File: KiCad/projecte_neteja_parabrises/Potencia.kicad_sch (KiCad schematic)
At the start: 10 parts

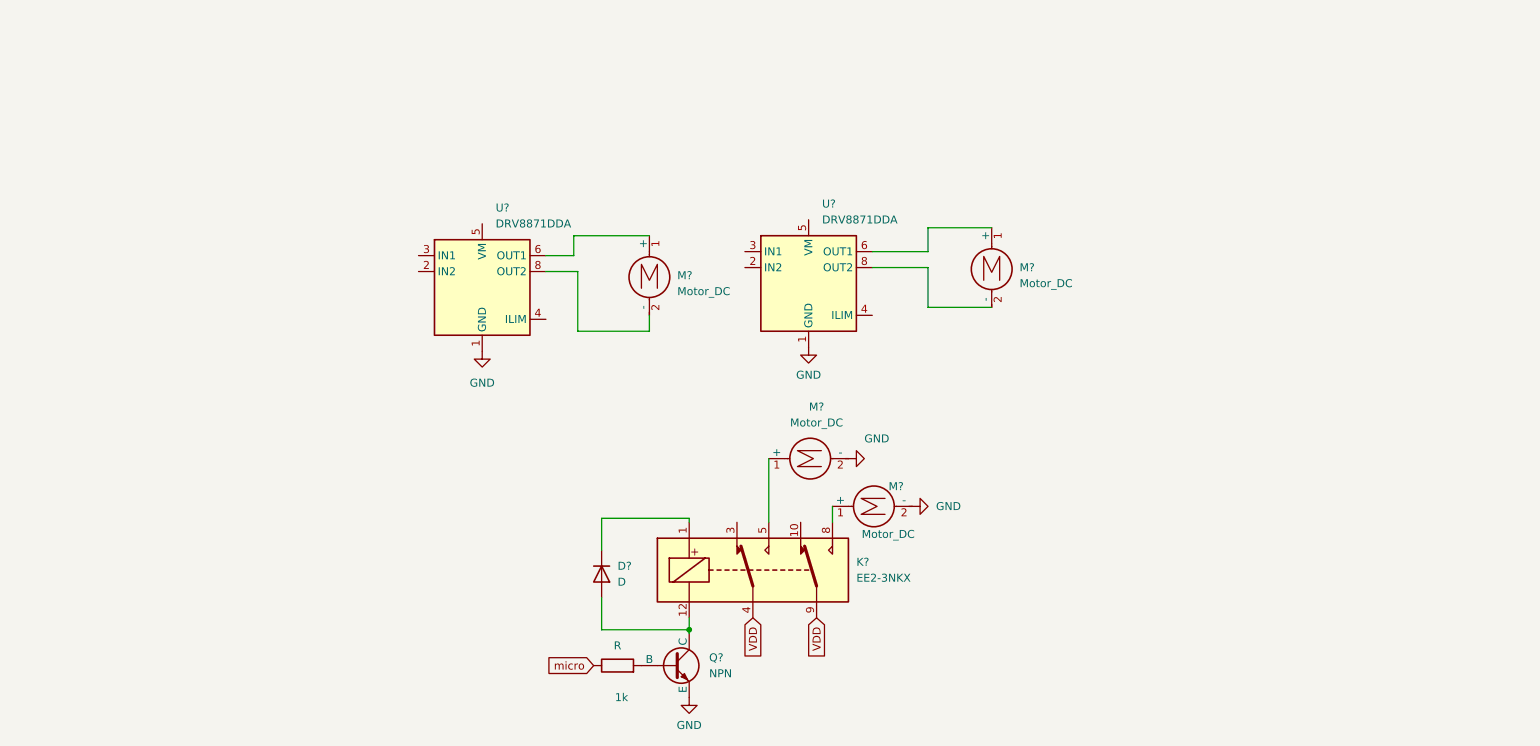
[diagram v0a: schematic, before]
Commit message: BOMBAS Y FINAL DEL CARRERA
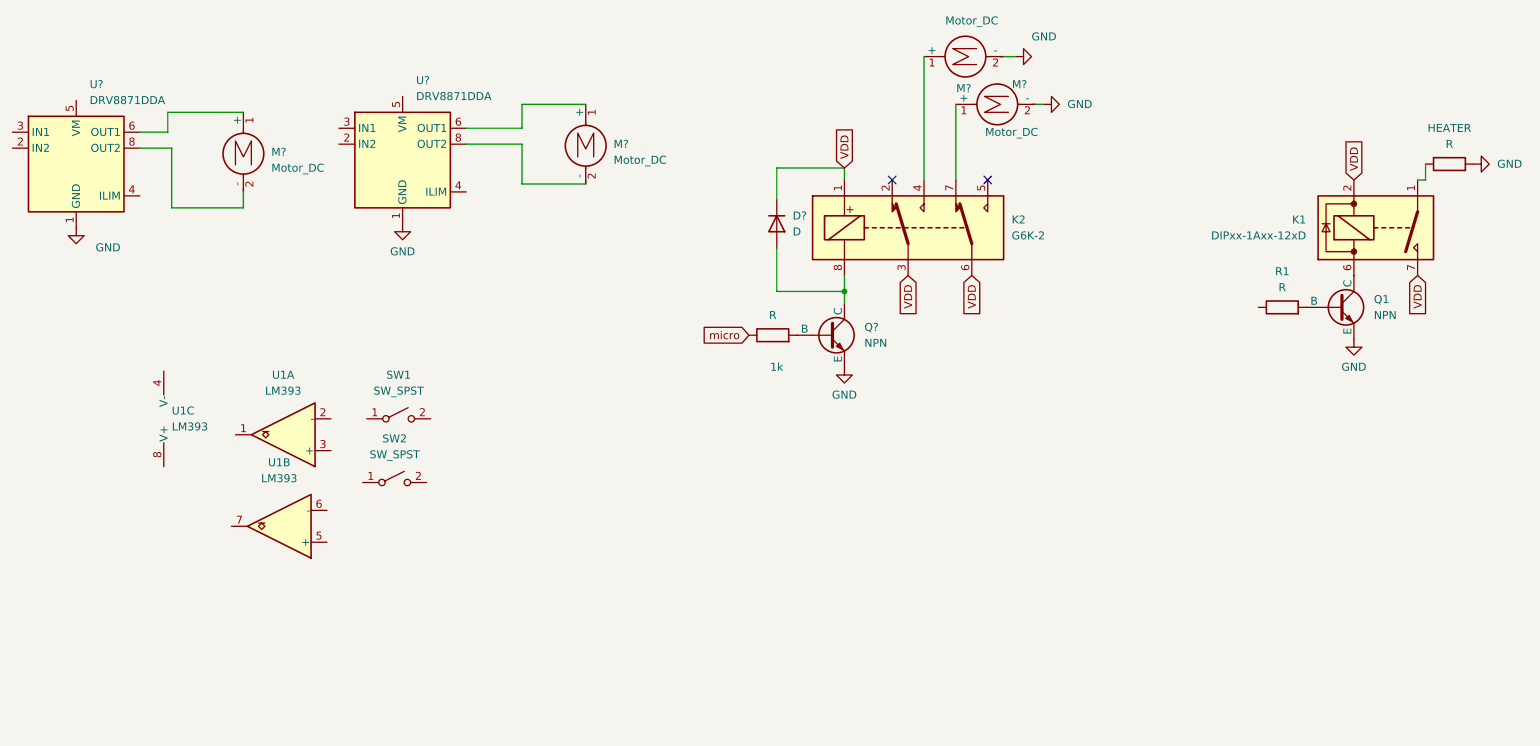
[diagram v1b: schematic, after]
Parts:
- removed K?: EE2-3NKX, Relay_SMD:Relay_DPDT_Kemet_EE2_NUX_NKX, symbol Relay:EE2-3NKX
- added HEATER, R1: R, symbol Device:R
- added K1: DIPxx-1Axx-12xD, Relay_THT:Relay_StandexMeder_DIP_LowProfile, symbol Relay:DIPxx-1Axx-12xD
- added K2: G6K-2, symbol Relay:G6K-2
- added Q1: NPN, symbol Simulation_SPICE:NPN
- added SW1, SW2: SW_SPST, symbol Switch:SW_SPST
- added U1: LM393, symbol Comparator:LM393
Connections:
- net GND: now also HEATER.2, Q1.3 (E)
- net VDD: now also D?.1 (K), K1.13, K1.2, K1.7, K1.8, K2.1, K2.3, K2.6
- net at D?.2 (A), Q?.1 (C): now also K2.8
- net at M?.1 (+): now also K2.7
- net at M?.1 (+): now also K2.4
- new net: Q1.2 (B), R1.2
- new net: HEATER.1, K1.1, K1.14
- new net: K1.6, Q1.1 (C)
- no-connect marks 0 -> 2
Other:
- moved on the sheet: 1k, D?, M?, Q?, U?
